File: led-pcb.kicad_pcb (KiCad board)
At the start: 2 copper layers, 100 x 40 mm, 142 parts, among them IC1 HT16K33A-28SSOP, J1 Conn_01x04_Pin

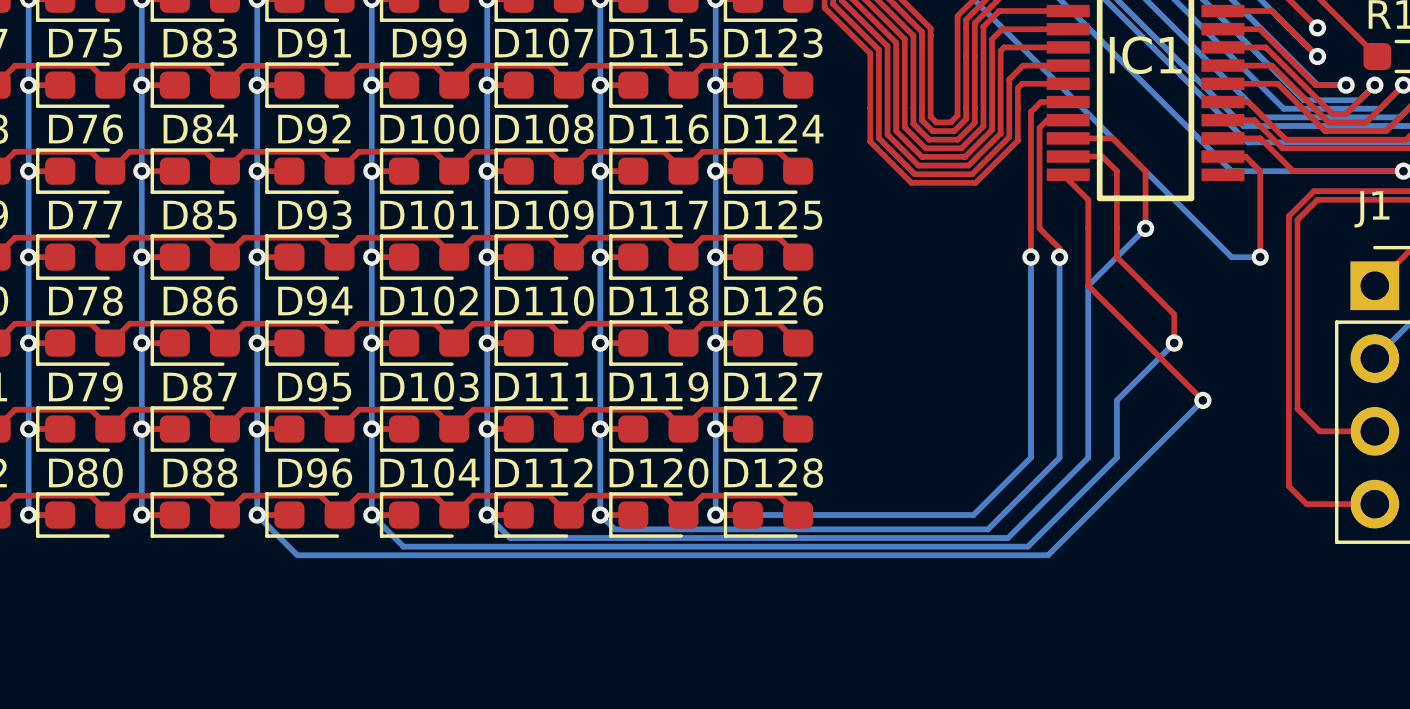
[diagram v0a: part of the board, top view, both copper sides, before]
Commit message: e
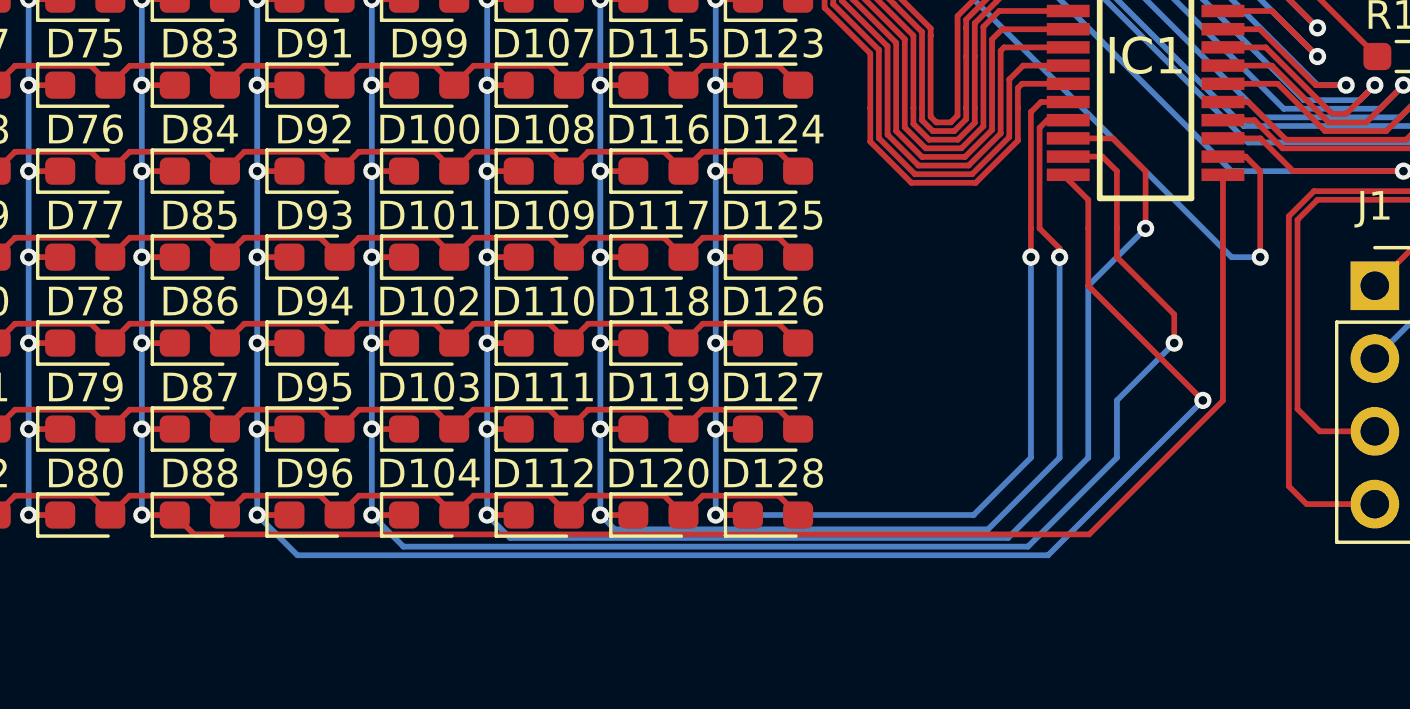
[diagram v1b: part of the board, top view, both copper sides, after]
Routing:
- net row10: track 30.4 -> 76.7 mm
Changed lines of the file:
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@@
 			(outputformat 1)
 			(mirror no)
-			(drillshape 1)
+			(drillshape 0)
 			(scaleselection 1)
 			(outputdirectory "")
@@
 	)
 	(segment
-		(start 179.7 110.128)
-		(end 180.128 110.128)
+		(start 143.801 122.676)
+		(end 143.125 122)
+		(width 0.2)
+		(layer "F.Cu")
+		(net 23)
+	)
+	(segment
+		(start 175.032521 122.676)
+		(end 143.801 122.676)
 		(width 0.2)
 		(layer "F.Cu")
@@
 	)
 	(segment
+		(start 179.7 110.128)
+		(end 179.7 118.008521)
+		(width 0.2)
+		(layer "F.Cu")
+		(net 23)
+	)
+	(segment
 		(start 143.1 119)
 		(end 141.975 119)
@@
 		(width 0.2)
 		(layer "F.Cu")
+		(net 23)
+	)
+	(segment
+		(start 179.7 118.008521)
+		(end 175.032521 122.676)
+		(width 0.2)
+		(layer "F.Cu")
